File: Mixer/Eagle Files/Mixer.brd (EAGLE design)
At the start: 94 x 59 mm, 50 parts, among them CON1 1-770875-01-770875-0_VERTICAL, IC1 LM741P, IC2 LM741P, T1 2N3904

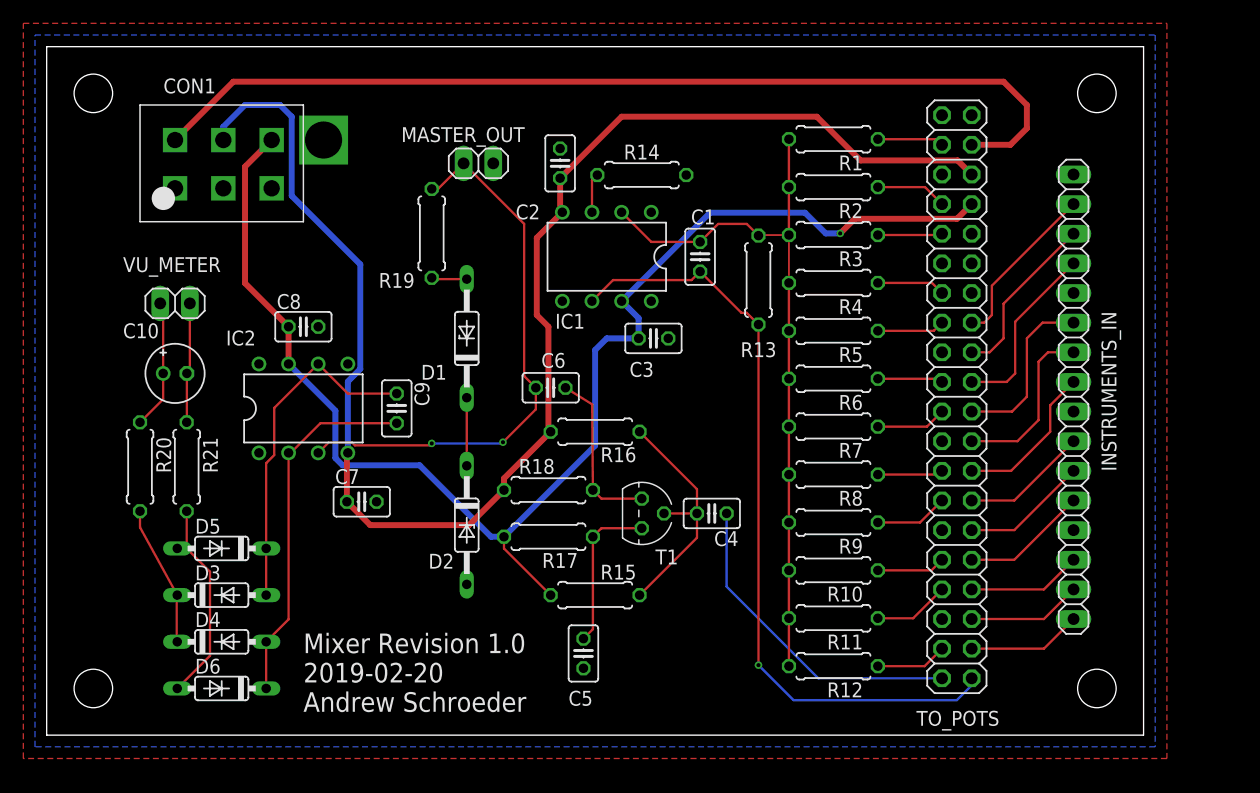
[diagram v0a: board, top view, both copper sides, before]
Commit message: Implemented changes from design review meeting.
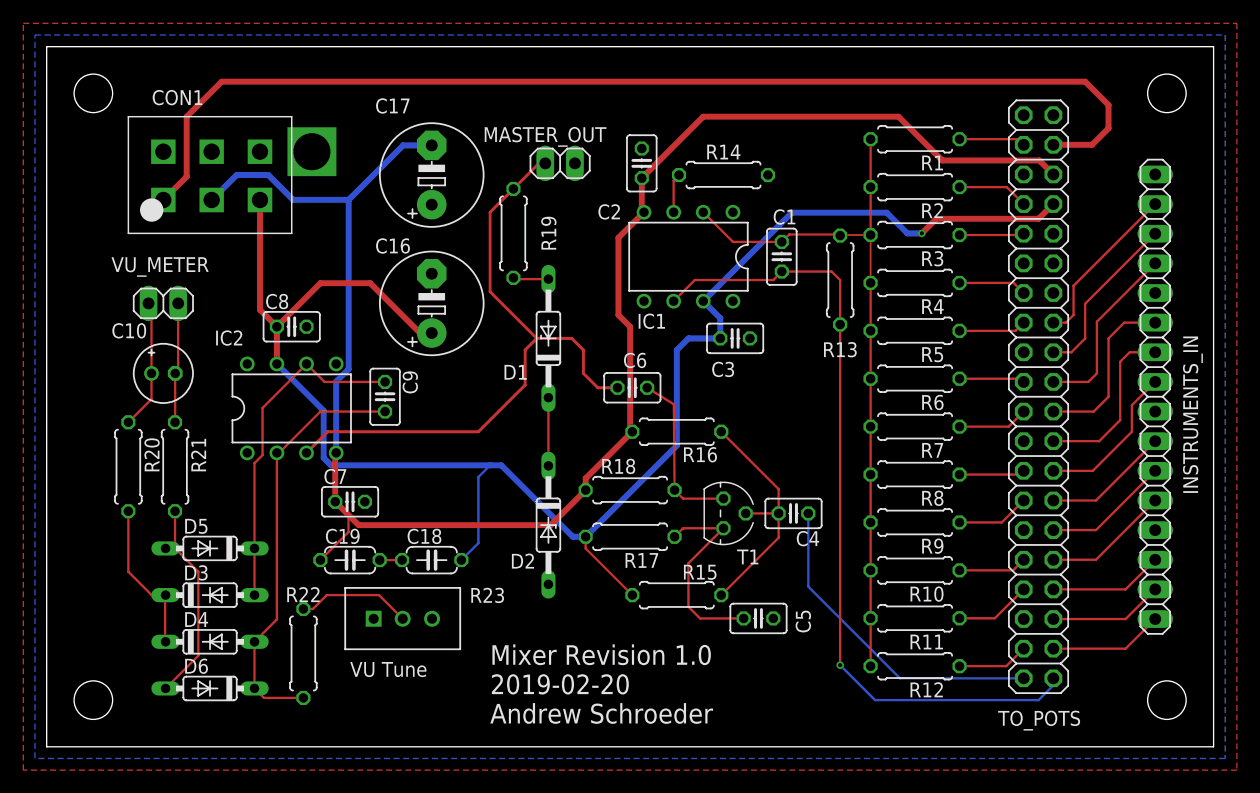
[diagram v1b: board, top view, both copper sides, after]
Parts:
- added C16, C17: 100uF, rcl:E5-8,5
- added C18, C19: 1u, resistor:C050-024X044
- added R22: 50, rcl:0207/7
- added R23: PV36W101C01B00, Capstone:POT_PV36W
- moved C5 15.3 mm to (61.0, 10.0), turned to 0 degrees
- moved C1 7.00 mm to (63.0, 41.0)
- moved C2 7.00 mm to (51.0, 49.0)
- moved C3 7.00 mm to (59.0, 34.0)
- moved C4 7.00 mm to (64.0, 19.0)
- moved C6 7.00 mm to (50.2, 29.8)
- moved D1 7.00 mm to (43.0, 34.0)
- moved D2 7.00 mm to (43.0, 18.0)
- moved IC1 7.00 mm to (55.0, 41.0)
- moved INSTRUMENTS_IN 7.00 mm to (95.0, 29.0)
- moved MASTER_OUT 7.00 mm to (44.0, 49.0)
- moved R1 7.00 mm to (74.4, 51.1)
- moved R10 7.00 mm to (74.4, 14.1)
- moved R11 7.00 mm to (74.4, 10.0)
- moved R12 7.00 mm to (74.4, 5.91)
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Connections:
- new net N$13: R22.1, R23.2
- net +12V: now also C16.+, C18.2
- net -12V: now also C17.-, C19.1
- net GND: now also C16.-, C17.+, C18.1, C19.2, R23.3; no longer CON1.3
- net N$3: now also R22.2
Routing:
- net +12V: track 117.4 -> 144.1 mm
- net -12V: track 129.0 -> 146.7 mm
- net +5V: track 83.2 -> 96.4 mm
- net N$13: track 0.00 -> 9.84 mm
- net SIG_OUT: track 47.7 -> 54.3 mm, vias 2 -> 0
- net N$3: track 31.4 -> 36.3 mm
- net N$8: track 13.6 -> 17.6 mm
- net MASTER_IN: track 67.0 -> 69.3 mm
- net GND: track 0.00 -> 1.92 mm
- net N$9: track 12.1 -> 13.4 mm
- net N$4: track 61.7 -> 61.0 mm
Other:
- board size 94 x 59 mm -> 100 x 60 mm
- board text added: "VU Tune"

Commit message: cleanup
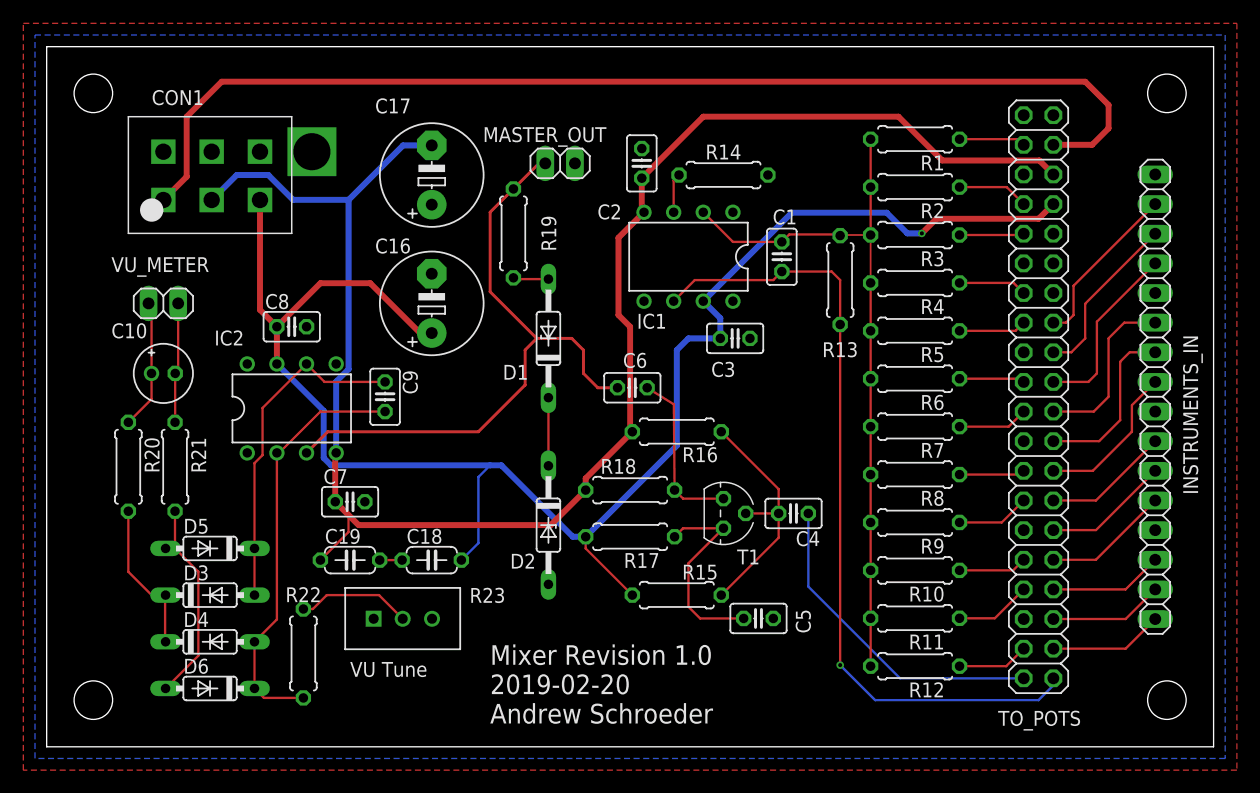
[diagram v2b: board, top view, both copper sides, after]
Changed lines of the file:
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@@
 <?xml version="1.0" encoding="utf-8"?>
 <!DOCTYPE eagle SYSTEM "eagle.dtd">
-<eagle version="9.2.2">
+<eagle version="9.3.1">
 <drawing>
 <settings>
@@
 </class>
 </classes>
-<designrules name="JLCPCB2Layer">
+<designrules name="SeeedStudio_2layer_DRU_no_angle_20140221">
 <description language="de">&lt;b&gt;EAGLE Design Rules&lt;/b&gt;
 &lt;p&gt;
@@
 </description>
 <param name="layerSetup" value="(1*16)"/>
-<param name="mtCopper" value="0.035mm 0.035mm 0.035mm 0.035mm 0.035mm 0.035mm 0.035mm 0.035mm 0.035mm 0.035mm 0.035mm 0.035mm 0.035mm 0.035mm 0.035mm 0.035mm"/>
-<param name="mtIsolate" value="1.5mm 0.15mm 0.2mm 0.15mm 0.2mm 0.15mm 0.2mm 0.15mm 0.2mm 0.15mm 0.2mm 0.15mm 0.2mm 0.15mm 0.2mm"/>
+<param name="mtCopper" value="0.035mm 0.0175mm 0.035mm 0.035mm 0.035mm 0.035mm 0.035mm 0.035mm 0.035mm 0.035mm 0.035mm 0.035mm 0.035mm 0.035mm 0.0175mm 0.035mm"/>
+<param name="mtIsolate" value="1.5mm 1.1mm 0.2mm 0.15mm 0.2mm 0.15mm 0.2mm 0.15mm 0.2mm 0.15mm 0.2mm 0.15mm 0.2mm 0.15mm 0.2mm"/>
 <param name="mdWireWire" value="6mil"/>
 <param name="mdWirePad" value="6mil"/>
@@
 <param name="mdSmdStop" value="0mil"/>
 <param name="msWidth" value="6mil"/>
-<param name="msDrill" value="10mil"/>
-<param name="msMicroVia" value="10mil"/>
+<param name="msDrill" value="12mil"/>
+<param name="msMicroVia" value="12mil"/>
 <param name="msBlindViaRatio" value="0.5"/>
 <param name="rvPadTop" value="0.25"/>
@@
 <param name="rvMicroViaOuter" value="0.25"/>
 <param name="rvMicroViaInner" value="0.25"/>
-<param name="rlMinPadTop" value="6mil"/>
+<param name="rlMinPadTop" value="10mil"/>
 <param name="rlMaxPadTop" value="20mil"/>
-<param name="rlMinPadInner" value="6mil"/>
+<param name="rlMinPadInner" value="10mil"/>
 <param name="rlMaxPadInner" value="20mil"/>
-<param name="rlMinPadBottom" value="6mil"/>
+<param name="rlMinPadBottom" value="10mil"/>
 <param name="rlMaxPadBottom" value="20mil"/>
 <param name="rlMinViaOuter" value="6mil"/>
